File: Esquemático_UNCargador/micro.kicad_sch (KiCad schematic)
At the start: 14 parts, among them J2 Relay, Q1 PN2222A, Q2 PN2222A

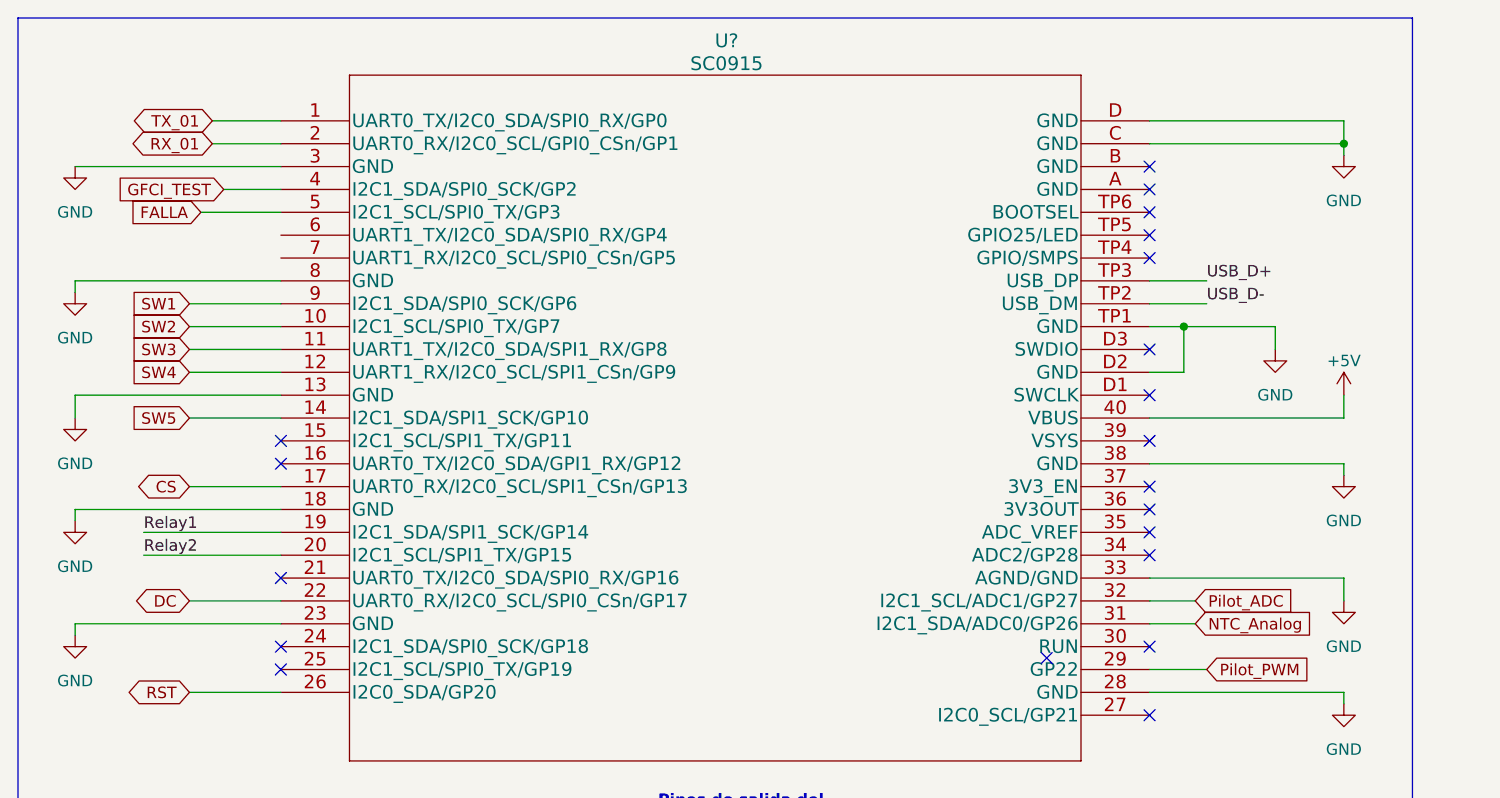
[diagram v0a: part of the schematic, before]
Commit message: Pinout sensores
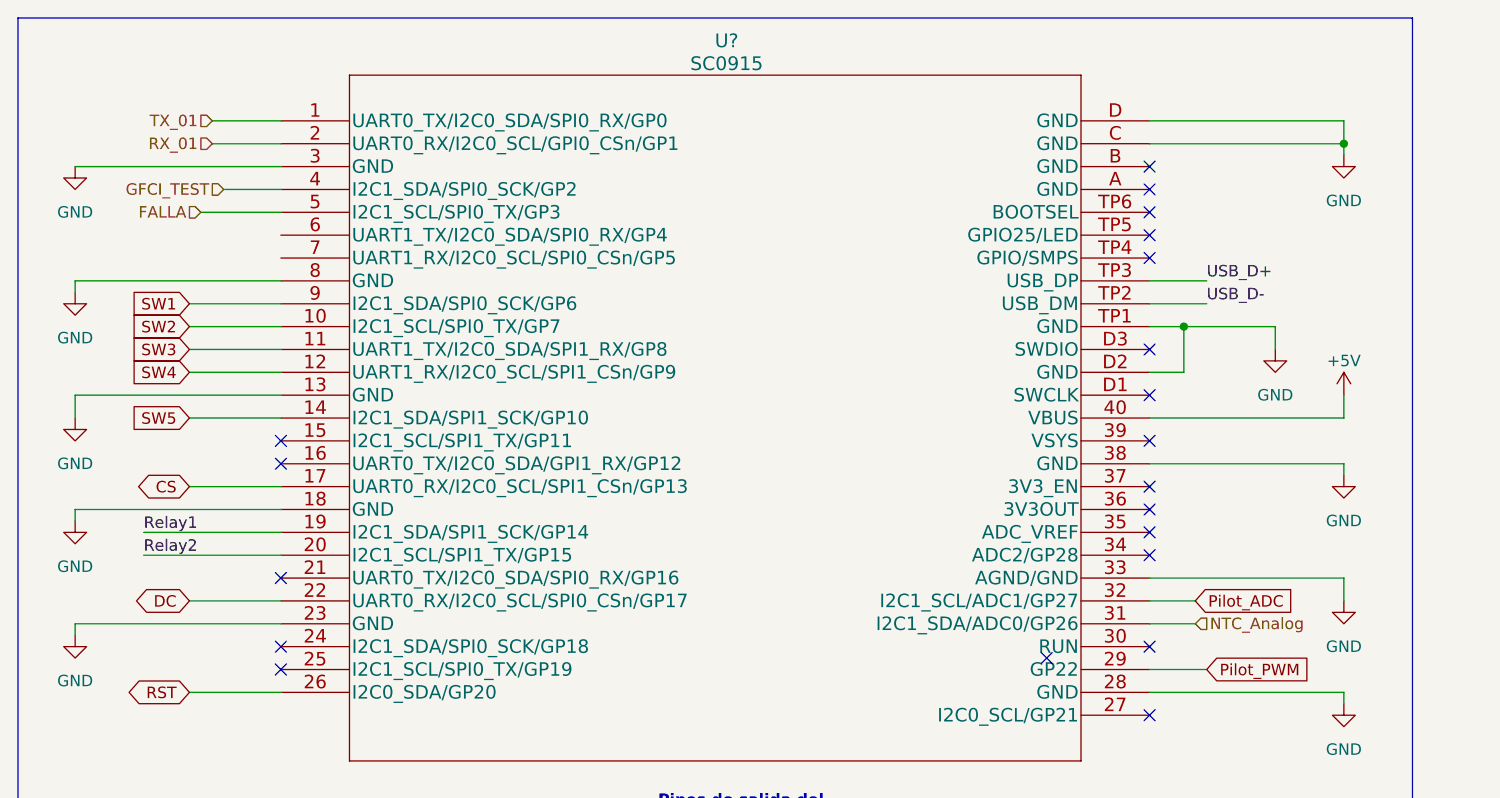
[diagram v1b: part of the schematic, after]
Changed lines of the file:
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@@
-    )
-  )
-  (global_label "NTC_Analog" (shape input) (at 154.94 91.44 0) (fields_autoplaced)
-    (effects (font (size 1.27 1.27)) (justify left))
-    (property "Intersheetrefs" "${INTERSHEET_REFS}" (at 168.7313 91.44 0)
-      (effects (font (size 1.27 1.27)) (justify left) hide)
     )
   )
@@
     )
   )
-  (global_label "RX_01" (shape bidirectional) (at 45.72 38.1 180) (fields_autoplaced)
-    (effects (font (size 1.27 1.27)) (justify right))
-    (property "Intersheetrefs" "${INTERSHEET_REFS}" (at 35.8368 38.1 0)
-      (effects (font (size 1.27 1.27)) (justify right) hide)
-    )
-  )
-  (global_label "FALLA" (shape input) (at 44.45 45.72 180) (fields_autoplaced)
-    (effects (font (size 1.27 1.27)) (justify right))
-    (property "Intersheetrefs" "${INTERSHEET_REFS}" (at 36.2222 45.72 0)
-      (effects (font (size 1.27 1.27)) (justify right) hide)
-    )
-  )
   (global_label "SW1" (shape input) (at 43.18 55.88 180) (fields_autoplaced)
     (effects (font (size 1.27 1.27)) (justify right))
@@
     (property "Intersheetrefs" "${INTERSHEET_REFS}" (at 61.3862 170.18 0)
       (effects (font (size 1.27 1.27)) (justify left) hide)
-    )
-  )
-  (global_label "TX_01" (shape bidirectional) (at 45.72 35.56 180) (fields_autoplaced)
-    (effects (font (size 1.27 1.27)) (justify right))
-    (property "Intersheetrefs" "${INTERSHEET_REFS}" (at 36.1392 35.56 0)
-      (effects (font (size 1.27 1.27)) (justify right) hide)
     )
   )
@@
     )
   )
-  (global_label "GFCI_TEST" (shape input) (at 46.99 43.18 180) (fields_autoplaced)
-    (effects (font (size 1.27 1.27)) (justify right))
-    (property "Intersheetrefs" "${INTERSHEET_REFS}" (at 34.5895 43.18 0)
-      (effects (font (size 1.27 1.27)) (justify right) hide)
-    )
-  )
   (global_label "CLK" (shape bidirectional) (at 125.73 160.02 0) (fields_autoplaced)
     (effects (font (size 1.27 1.27)) (justify left))
@@
     )
   )
+  (hierarchical_label "FALLA" (shape input) (at 44.45 45.72 180) (fields_autoplaced)
+    (effects (font (size 1.27 1.27)) (justify right))
+  )
+  (hierarchical_label "NTC_Analog" (shape input) (at 154.94 91.44 0) (fields_autoplaced)
+    (effects (font (size 1.27 1.27)) (justify left))
+  )
+  (hierarchical_label "RX_01" (shape input) (at 45.72 38.1 180) (fields_autoplaced)
+    (effects (font (size 1.27 1.27)) (justify right))
+  )
+  (hierarchical_label "TX_01" (shape input) (at 45.72 35.56 180) (fields_autoplaced)
+    (effects (font (size 1.27 1.27)) (justify right))
+  )
+  (hierarchical_label "GFCI_TEST" (shape input) (at 46.99 43.18 180) (fields_autoplaced)
+    (effects (font (size 1.27 1.27)) (justify right))
+  )
   (symbol (lib_id "Switch:SW_Push") (at 46.99 143.51 0) (unit 1)
